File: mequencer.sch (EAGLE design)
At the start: 75 parts, among them IC1 NE555D, IC10 LF353D, IC11 NE555D, IC12 NE555D, IC2 4163D, IC3 74HC85D, IC4 4051D, IC5 4051D, IC6 74HCT04D, IC7 4051D, IC8 4051D, IC9 LF353D, U1 74LVC1G08SE-7

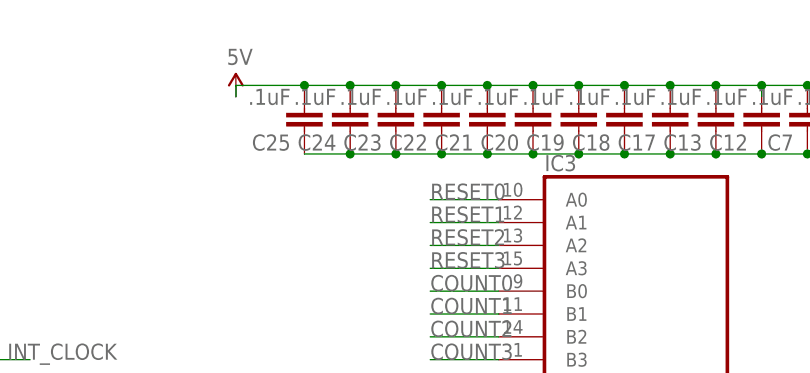
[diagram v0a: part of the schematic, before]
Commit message: Moving shit around more
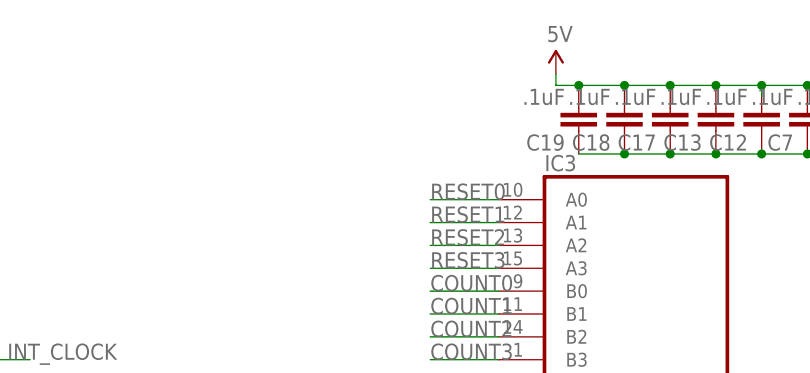
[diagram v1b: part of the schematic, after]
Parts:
- removed C20, C21, C22, C23, C24, C25: .1uF, SparkFun-Capacitors:CAP0603-CAP
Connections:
- net 5V: no longer C20.2, C21.2, C22.2, C23.2, C24.2, C25.2
- net N$7: no longer C20.1, C21.1, C22.1, C23.1, C24.1, C25.1
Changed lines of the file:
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@@
 <part name="C18" library="SparkFun-Capacitors" deviceset="CAP" device="0603-CAP" value=".1uF"/>
 <part name="C19" library="SparkFun-Capacitors" deviceset="CAP" device="0603-CAP" value=".1uF"/>
-<part name="C20" library="SparkFun-Capacitors" deviceset="CAP" device="0603-CAP" value=".1uF"/>
-<part name="C21" library="SparkFun-Capacitors" deviceset="CAP" device="0603-CAP" value=".1uF"/>
-<part name="C22" library="SparkFun-Capacitors" deviceset="CAP" device="0603-CAP" value=".1uF"/>
-<part name="C23" library="SparkFun-Capacitors" deviceset="CAP" device="0603-CAP" value=".1uF"/>
-<part name="C24" library="SparkFun-Capacitors" deviceset="CAP" device="0603-CAP" value=".1uF"/>
-<part name="C25" library="SparkFun-Capacitors" deviceset="CAP" device="0603-CAP" value=".1uF"/>
 <part name="R2" library="SparkFun-Resistors" deviceset="RESISTOR" device="0603" value="1k"/>
 <part name="JP2" library="SparkFun-Connectors" deviceset="M04" device="JST-PTH"/>
@@
 <instance part="C5" gate="G$1" x="26.67" y="173.99" rot="R180"/>
 <instance part="C6" gate="G$1" x="55.88" y="172.72" rot="R180"/>
-<instance part="SUPPLY13" gate="G$1" x="92.71" y="181.61"/>
+<instance part="SUPPLY13" gate="G$1" x="128.27" y="184.15"/>
 <instance part="GND4" gate="1" x="237.49" y="100.33"/>
 <instance part="C7" gate="G$1" x="156.21" y="180.34" rot="R180"/>
@@
 <instance part="C18" gate="G$1" x="135.89" y="180.34" rot="R180"/>
 <instance part="C19" gate="G$1" x="130.81" y="180.34" rot="R180"/>
-<instance part="C20" gate="G$1" x="125.73" y="180.34" rot="R180"/>
-<instance part="C21" gate="G$1" x="120.65" y="180.34" rot="R180"/>
-<instance part="C22" gate="G$1" x="115.57" y="180.34" rot="R180"/>
-<instance part="C23" gate="G$1" x="110.49" y="180.34" rot="R180"/>
-<instance part="C24" gate="G$1" x="105.41" y="180.34" rot="R180"/>
-<instance part="C25" gate="G$1" x="100.33" y="180.34" rot="R180"/>
 <instance part="R2" gate="G$1" x="25.4" y="149.86"/>
 <instance part="JP2" gate="G$1" x="10.16" y="-15.24"/>
@@
 </segment>
 <segment>
-<pinref part="C25" gate="G$1" pin="2"/>
-<pinref part="C24" gate="G$1" pin="2"/>
-<wire x1="100.33" y1="182.88" x2="105.41" y2="182.88" width="0.1524" layer="91"/>
-<pinref part="C23" gate="G$1" pin="2"/>
-<wire x1="105.41" y1="182.88" x2="110.49" y2="182.88" width="0.1524" layer="91"/>
-<junction x="105.41" y="182.88"/>
-<pinref part="C22" gate="G$1" pin="2"/>
-<wire x1="110.49" y1="182.88" x2="115.57" y2="182.88" width="0.1524" layer="91"/>
-<junction x="110.49" y="182.88"/>
-<pinref part="C21" gate="G$1" pin="2"/>
-<wire x1="115.57" y1="182.88" x2="120.65" y2="182.88" width="0.1524" layer="91"/>
-<junction x="115.57" y="182.88"/>
-<pinref part="C20" gate="G$1" pin="2"/>
-<wire x1="120.65" y1="182.88" x2="125.73" y2="182.88" width="0.1524" layer="91"/>
-<junction x="120.65" y="182.88"/>
 <pinref part="C19" gate="G$1" pin="2"/>
-<wire x1="125.73" y1="182.88" x2="130.81" y2="182.88" width="0.1524" layer="91"/>
-<junction x="125.73" y="182.88"/>
+<wire x1="128.27" y1="182.88" x2="130.81" y2="182.88" width="0.1524" layer="91"/>
 <pinref part="C18" gate="G$1" pin="2"/>
 <wire x1="130.81" y1="182.88" x2="135.89" y2="182.88" width="0.1524" layer="91"/>
@@
 <junction x="186.69" y="182.88"/>
 <pinref part="SUPPLY13" gate="G$1" pin="5V"/>
-<wire x1="100.33" y1="182.88" x2="92.71" y2="182.88" width="0.1524" layer="91"/>
-<wire x1="92.71" y1="182.88" x2="92.71" y2="181.61" width="0.1524" layer="91"/>
-<junction x="100.33" y="182.88"/>
+<wire x1="128.27" y1="182.88" x2="128.27" y2="184.15" width="0.1524" layer="91"/>
 </segment>
 <segment>
@@
 <wire x1="208.28" y1="124.46" x2="223.52" y2="124.46" width="0.1524" layer="91"/>
 <junction x="223.52" y="124.46"/>
-<pinref part="C25" gate="G$1" pin="1"/>
-<pinref part="C24" gate="G$1" pin="1"/>
-<wire x1="100.33" y1="175.26" x2="105.41" y2="175.26" width="0.1524" layer="91"/>
-<pinref part="C23" gate="G$1" pin="1"/>
-<wire x1="105.41" y1="175.26" x2="110.49" y2="175.26" width="0.1524" layer="91"/>
-<junction x="105.41" y="175.26"/>
-<pinref part="C22" gate="G$1" pin="1"/>
-<wire x1="110.49" y1="175.26" x2="115.57" y2="175.26" width="0.1524" layer="91"/>
-<junction x="110.49" y="175.26"/>
-<pinref part="C21" gate="G$1" pin="1"/>
-<wire x1="115.57" y1="175.26" x2="120.65" y2="175.26" width="0.1524" layer="91"/>
-<junction x="115.57" y="175.26"/>
-<pinref part="C20" gate="G$1" pin="1"/>
-<wire x1="120.65" y1="175.26" x2="125.73" y2="175.26" width="0.1524" layer="91"/>
-<junction x="120.65" y="175.26"/>
 <pinref part="C19" gate="G$1" pin="1"/>
-<wire x1="125.73" y1="175.26" x2="130.81" y2="175.26" width="0.1524" layer="91"/>
-<junction x="125.73" y="175.26"/>
 <pinref part="C18" gate="G$1" pin="1"/>
 <wire x1="130.81" y1="175.26" x2="135.89" y2="175.26" width="0.1524" layer="91"/>
-<junction x="130.81" y="175.26"/>
 <pinref part="C17" gate="G$1" pin="1"/>
 <wire x1="135.89" y1="175.26" x2="140.97" y2="175.26" width="0.1524" layer="91"/>
